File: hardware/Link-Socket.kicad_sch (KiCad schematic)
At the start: 4 parts, among them J1901 2x05_Horizontal, U1901 THVD2442

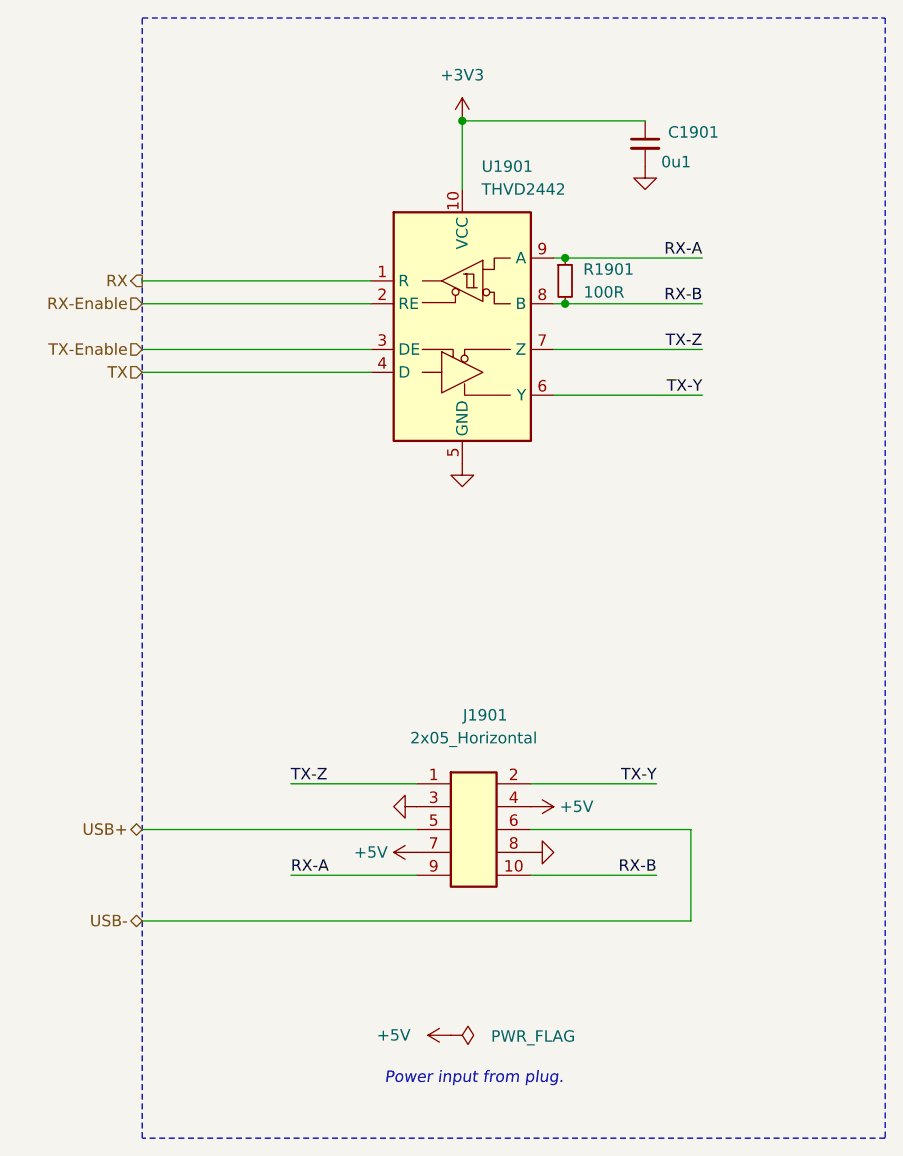
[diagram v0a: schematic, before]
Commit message: Rename
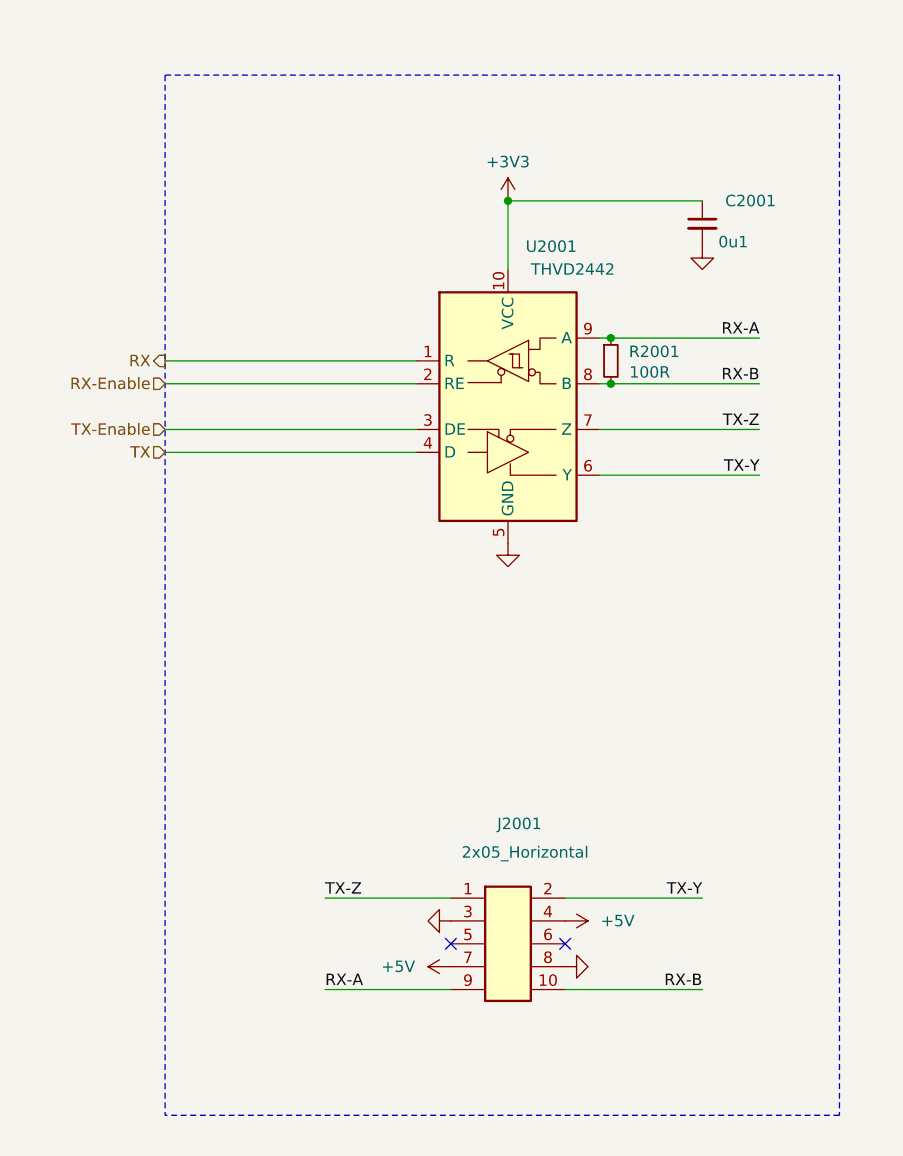
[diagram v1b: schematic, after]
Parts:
- removed C1901: 0u1, V2_Capacitor_SMD:C_1608, symbol V2_Capacitor:1608_0u1
- removed J1901: 2x05_Horizontal, V2_Connector_Header_1.27mm:PinHeader_2x05_P1.27mm_Horizontal, symbol V2_Connector_Header_1.27mm:2x05_Horizontal
- removed R1901: 100R, V2_Resistor_SMD:R_1608, symbol V2_Resistor:1608_100R
- removed U1901: THVD2442, V2_Package_SON:VSON-10-4-1EP_3x3mm_P0.5mm_EP1.65x2.4mm_ThermalVias, symbol V2_Interface_RS485:THVD2442
- added C2001: 0u1, V2_Capacitor_SMD:C_1608, symbol V2_Capacitor:1608_0u1
- added J2001: 2x05_Horizontal, V2_Connector_Header_1.27mm:PinHeader_2x05_P1.27mm_Horizontal, symbol V2_Connector_Header_1.27mm:2x05_Horizontal
- added R2001: 100R, V2_Resistor_SMD:R_1608, symbol V2_Resistor:1608_100R
- added U2001: THVD2442, V2_Package_SON:VSON-10-4-1EP_3x3mm_P0.5mm_EP1.65x2.4mm_ThermalVias, symbol V2_Interface_RS485:THVD2442
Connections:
- net +3V3: now also C2001.1, U2001.10 (VCC)
- net +5V: now also J2001.4 (Pin_4), J2001.7 (Pin_7)
- net GND: now also C2001.2, J2001.3 (Pin_3), J2001.8 (Pin_8), U2001.11 (GND), U2001.5 (GND)
- net RX: now also U2001.1 (R)
- net RX-A: now also J2001.9 (Pin_9), R2001.1, U2001.9 (A)
- net RX-B: now also J2001.10 (Pin_10), R2001.2, U2001.8 (B)
- net RX-Enable: now also U2001.2 (RE)
- net TX: now also U2001.4 (D)
- net TX-Enable: now also U2001.3 (DE)
- net TX-Y: now also J2001.2 (Pin_2), U2001.6 (Y)
- net TX-Z: now also J2001.1 (Pin_1), U2001.7 (Z)
- no-connect marks 0 -> 2
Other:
- note removed: "Power input from plug."
